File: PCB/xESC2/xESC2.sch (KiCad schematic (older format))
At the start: 4 parts

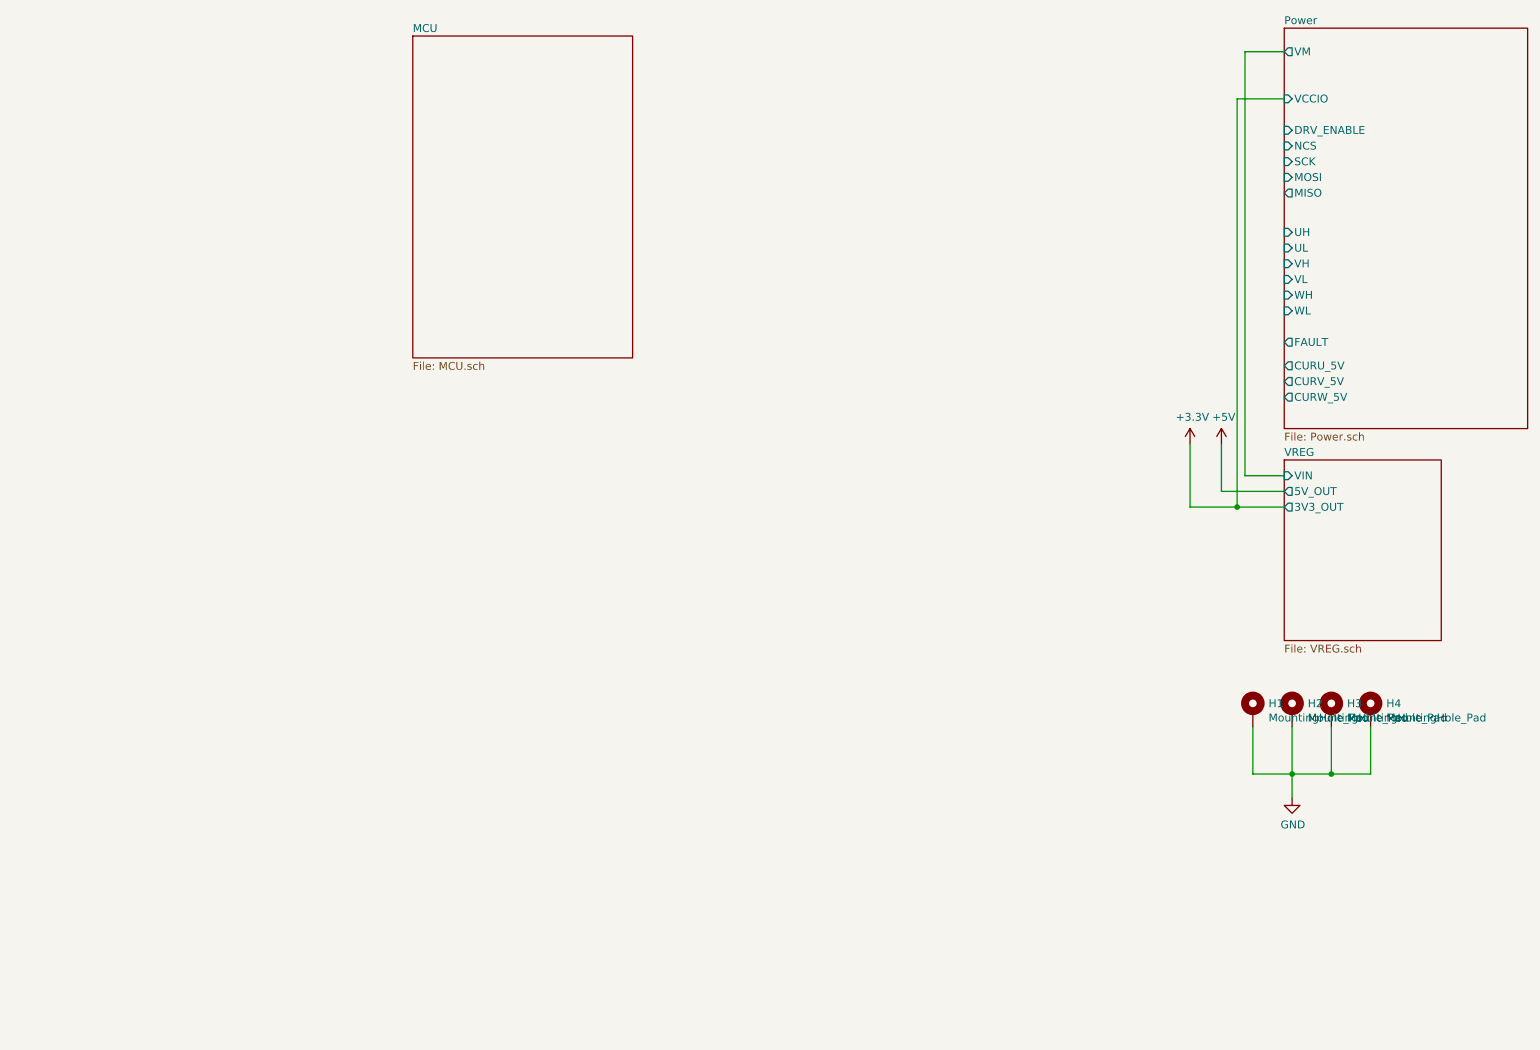
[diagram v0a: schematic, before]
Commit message: wip logic
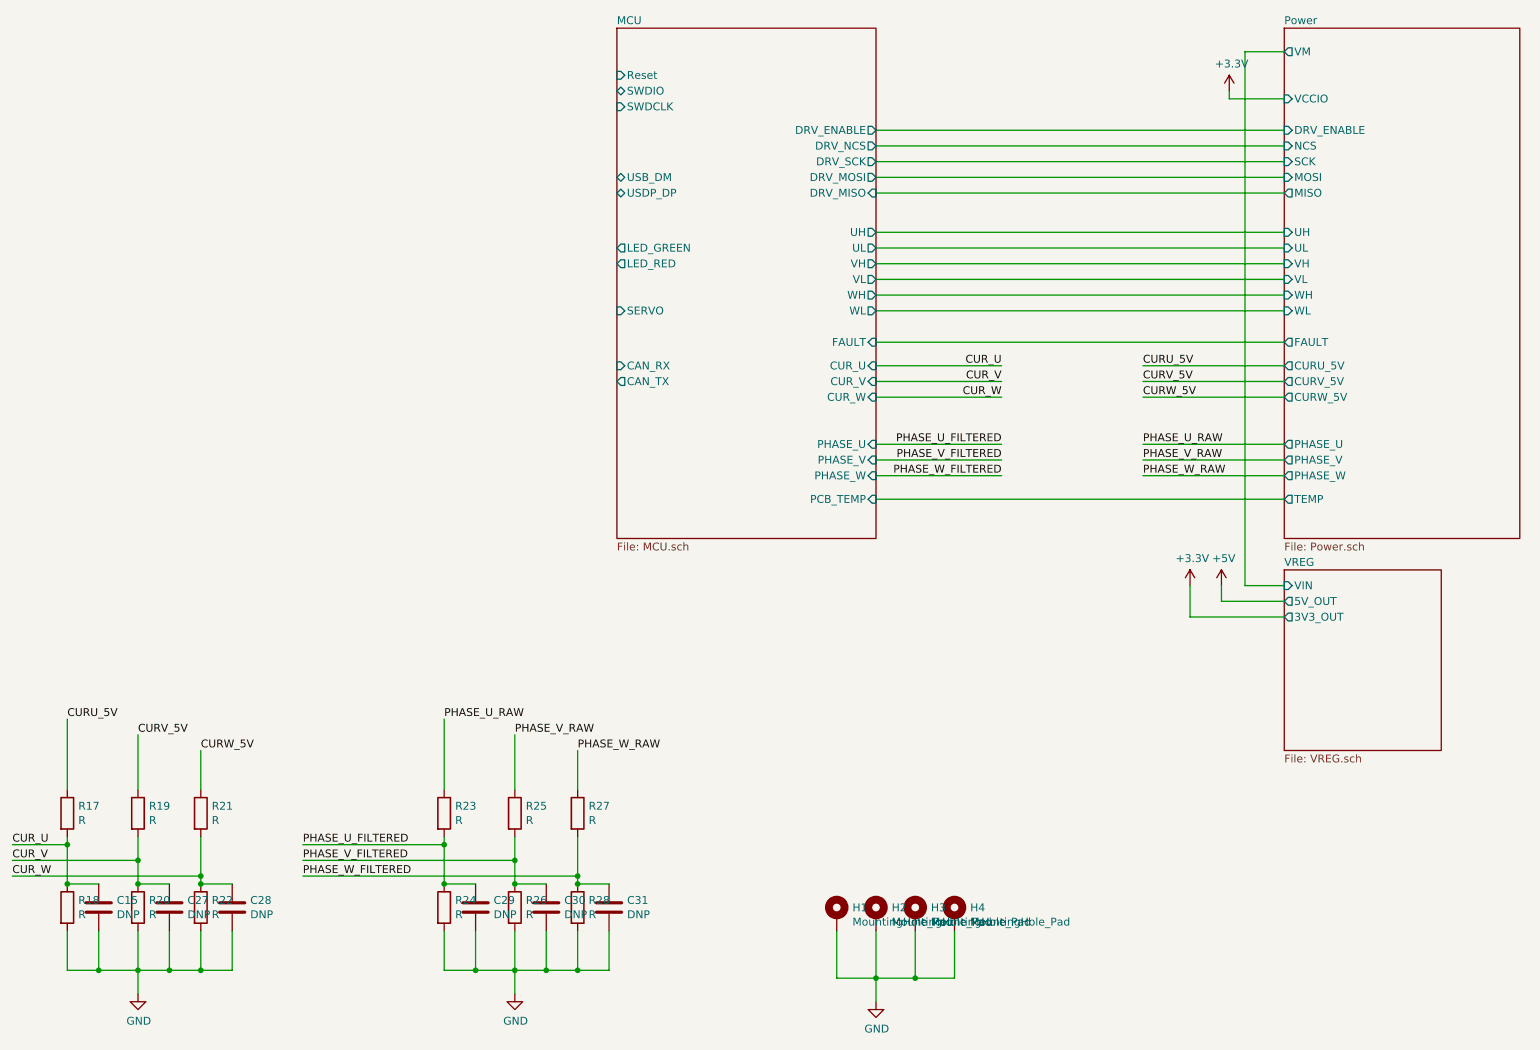
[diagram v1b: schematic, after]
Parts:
- added C15, C27, C28, C29, C30, C31: DNP, Capacitor_SMD:C_0603_1608Metric, symbol Device:C
- added R17, R18, R19, R20, R21, R22, R23, R24, R25, R26, R27, R28: R, Resistor_SMD:R_0603_1608Metric, symbol Device:R
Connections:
- net GND: now also C15.2, C27.2, C28.2, C29.2, C30.2, C31.2, R18.2, R20.2, R22.2, R24.2, R26.2, R28.2
- new net CURU_5V: R17.1
- new net CURV_5V: R19.1
- new net CURW_5V: R21.1
- new net CUR_U: C15.1, R17.2, R18.1
- new net CUR_V: C27.1, R19.2, R20.1
- new net CUR_W: C28.1, R21.2, R22.1
- new net PHASE_U_FILTERED: C29.1, R23.2, R24.1
- new net PHASE_U_RAW: R23.1
- new net PHASE_V_FILTERED: C30.1, R25.2, R26.1
- new net PHASE_V_RAW: R25.1
- new net PHASE_W_FILTERED: C31.1, R27.2, R28.1
- new net PHASE_W_RAW: R27.1
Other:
- moved on the sheet: H1, H2, H3, H4
